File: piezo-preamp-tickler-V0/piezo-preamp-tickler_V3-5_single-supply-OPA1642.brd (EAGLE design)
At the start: 100.3 x 20.1 mm, 58 parts, among them IC1 OPA1642, IC2 DMN2400, IC3 BQ21040, IC4 BQ297X, IC5 SC4503, IC6 TPS7A49, J1 HEADPHONES, J2 PHONE, J3 Mixer, J5 Battery, Q1 MMBFJ201, SW1 SWITCH_DPDT, SW2 INPUT-select, SW3 SPDT

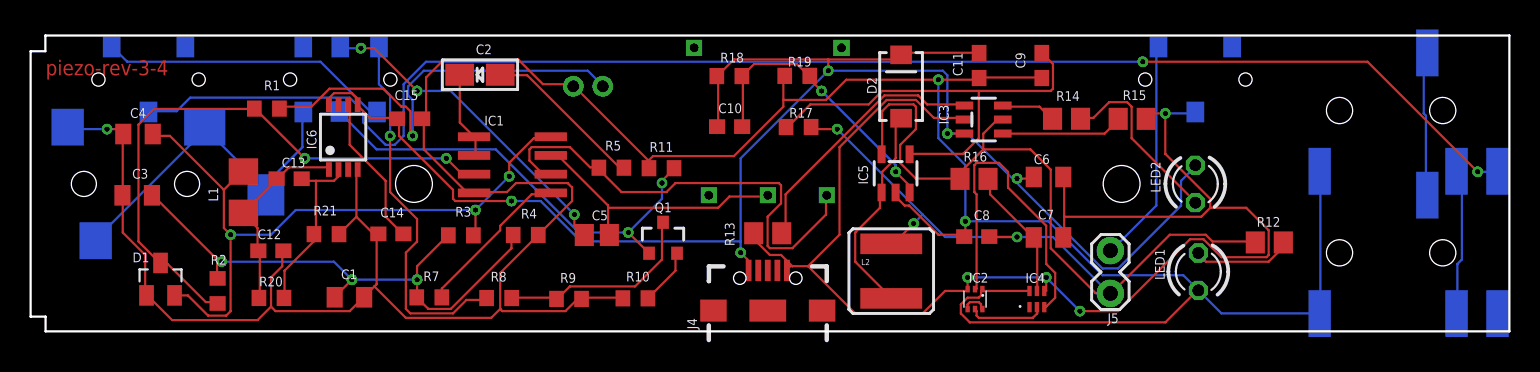
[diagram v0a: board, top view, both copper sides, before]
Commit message: boards layed out
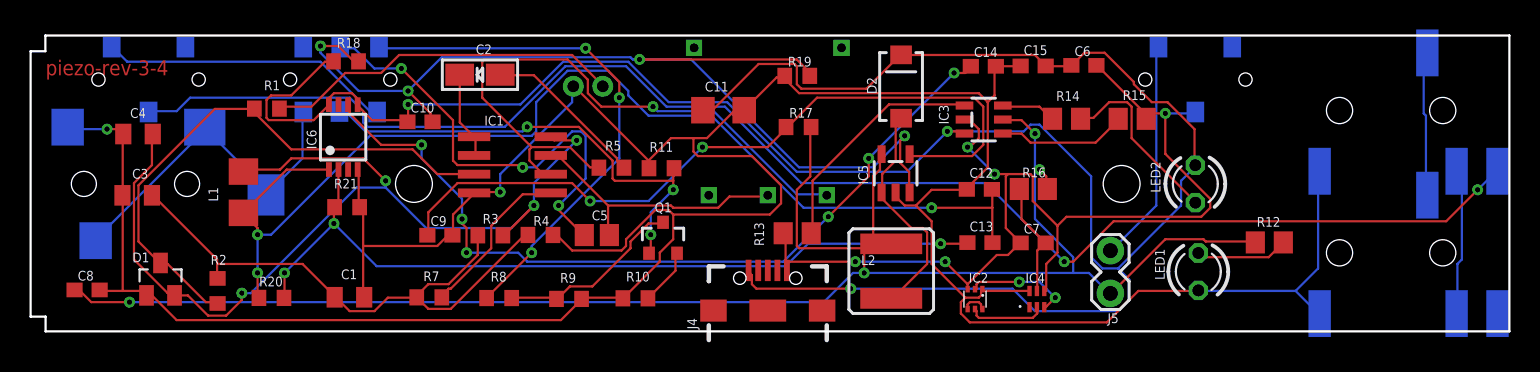
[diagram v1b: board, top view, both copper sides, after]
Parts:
- C10: value 2.2pf -> 2.2pF; device adafruit:C0603 -> rcl:C0603
- C11: device adafruit:C0603 -> rcl:C1206
- C12, C13, C14, C15, C8: device adafruit:C0603 -> rcl:C0603
- C6, C7: device adafruit:C0805K -> rcl:C0603
- C9: value 56nf -> 56nF; device adafruit:C0603 -> rcl:C0603
- moved C8 60.5 mm to (3.83, 2.81), turned to 0 degrees
- moved C12 48.2 mm to (64.3, 9.63), turned to 180 degrees
- moved C13 47.1 mm to (64.4, 6.02), turned to 180 degrees
- moved C15 42.4 mm to (68.0, 18.0), turned to 180 degrees
- moved C9 42.4 mm to (27.8, 6.52), turned to 0 degrees
- moved C14 41.8 mm to (64.6, 18.0), turned to 0 degrees
- moved R18 26.0 mm to (21.4, 18.3)
- moved C10 21.0 mm to (26.4, 14.2)
- moved C11 17.6 mm to (47.0, 15.0), turned to 0 degrees
- moved C6 7.94 mm to (71.4, 18.0)
- moved R16 4.08 mm to (68.0, 9.66), turned to 180 degrees
- moved R21 2.30 mm to (21.5, 8.42)
- moved R13 2.00 mm to (52.0, 6.66)
- moved R3 2.00 mm to (31.2, 6.51)
- moved C7 1.10 mm to (68.0, 6.00)
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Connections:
- net GND2: now also C7.1; no longer C7.2
- net N$42: now also C7.2; no longer C7.1
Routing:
- net +12V: track 13.4 -> 76.5 mm, vias 0 -> 3
- net V+: track 112.2 -> 163.8 mm, vias 5 -> 3
- net N$30: track 19.5 -> 68.3 mm, vias 2 -> 4
- net VBAT: track 77.0 -> 124.9 mm, vias 3 -> 4
- net N$28: track 10.3 -> 55.7 mm, vias 0 -> 6
- net N$26: track 12.0 -> 55.1 mm, vias 0 -> 3
- net GND2: track 95.1 -> 70.9 mm, vias 4 -> 5
- net N$29: track 30.3 -> 51.7 mm, vias 0 -> 2
- net N$25: track 48.0 -> 65.0 mm, vias 3 -> 4
- net N$45: track 22.0 -> 7.25 mm, vias 0 -> 2
- net N$7: track 32.1 -> 42.9 mm, vias 0 -> 1
- net N$11: track 25.2 -> 35.6 mm, vias 1 -> 3
- net N$16: track 22.3 -> 31.0 mm
- net GND: track 220.8 -> 215.1 mm, vias 3 -> 2
- net N$2: track 29.4 -> 24.4 mm, vias 1 -> 0
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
